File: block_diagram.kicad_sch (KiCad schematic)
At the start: 0 parts

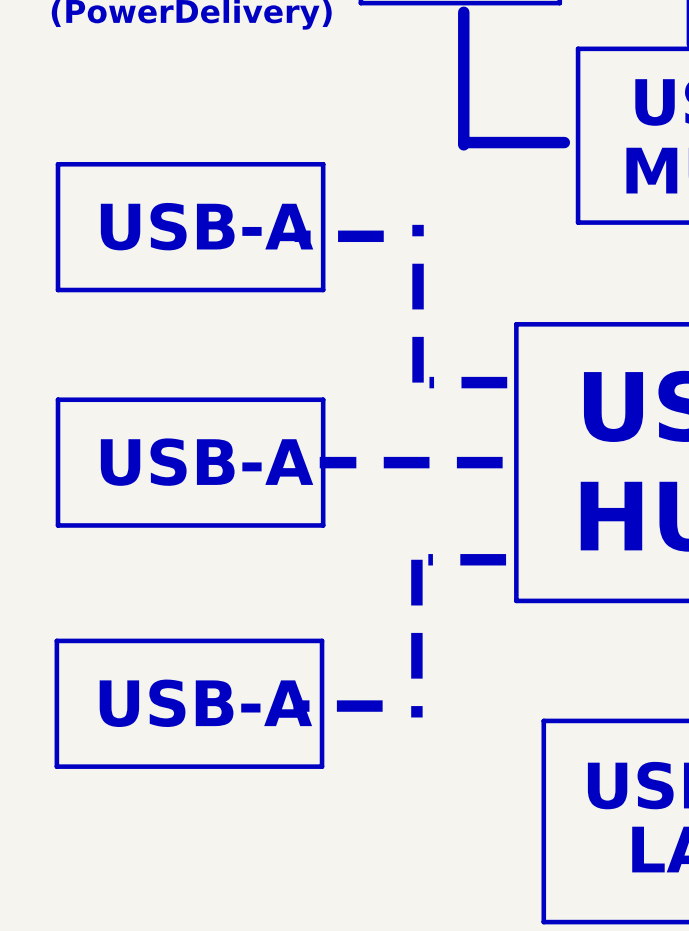
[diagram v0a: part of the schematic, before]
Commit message: Add files via upload
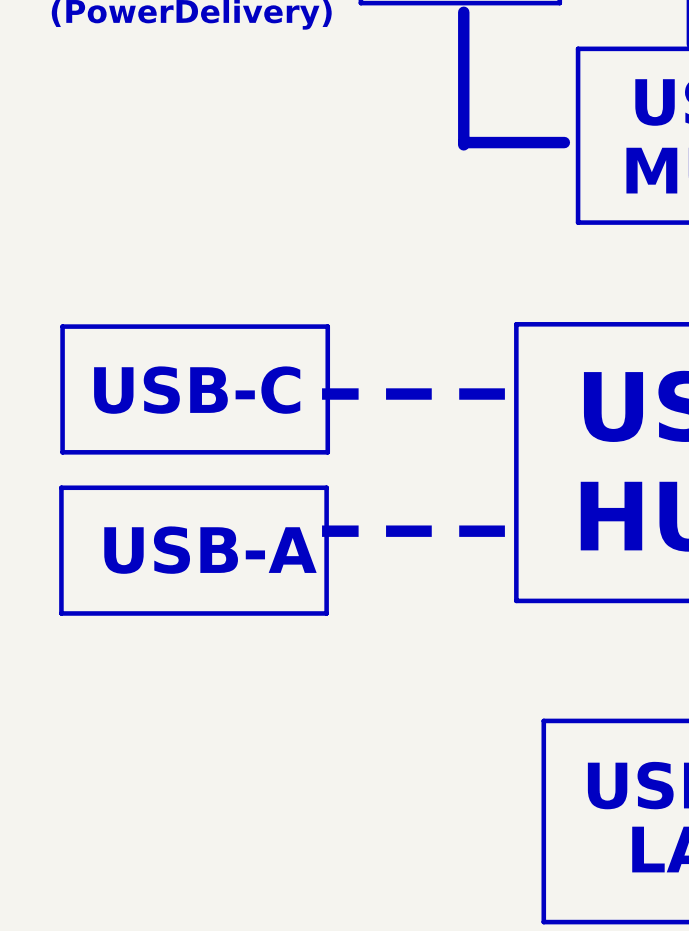
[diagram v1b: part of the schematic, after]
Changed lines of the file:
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@@
-	)
-	(rectangle
-		(start 62.103 84.963)
-		(end 91.567 98.933)
-		(stroke
-			(width 0.508)
-			(type solid)
-			(color 221 133 0 1)
-		)
-		(fill
-			(type none)
-		)
 	)
 	(rectangle
@@
 	)
 	(rectangle
-		(start 61.976 137.922)
-		(end 91.44 151.892)
+		(start 62.484 120.904)
+		(end 91.948 134.874)
 		(stroke
 			(width 0.508)
@@
 	)
 	(rectangle
-		(start 62.103 111.125)
-		(end 91.567 125.095)
+		(start 62.611 102.997)
+		(end 92.075 116.967)
 		(stroke
 			(width 0.508)
@@
 		)
 	)
+	(text "USB-C"
+		(exclude_from_sim no)
+		(at 77.47 110.49 0)
+		(effects
+			(font
+				(size 5.08 5.08)
+				(thickness 1.016)
+				(bold yes)
+				(color 221 133 0 1)
+			)
+		)
+	)
+	(text "HUB"
+		(exclude_from_sim no)
+		(at 131.826 124.587 0)
+		(effects
+			(font
+				(size 7.62 7.62)
+				(thickness 1.524)
+				(bold yes)
+				(color 255 153 0 1)
+			)
+		)
+	)
+	(text "LAN"
+		(exclude_from_sim no)
+		(at 133.096 161.544 0)
+		(effects
+			(font
+				(size 5.08 5.08)
+				(thickness 1.016)
+				(bold yes)
+				(color 132 0 132 1)
+			)
+		)
+	)
 	(text "USB-A "
 		(exclude_from_sim no)
-		(at 78.359 118.491 0)
-		(effects
-			(font
-				(size 5.08 5.08)
-				(thickness 1.016)
-				(bold yes)
-				(color 221 133 0 1)
-			)
-		)
-	)
-	(text "HUB"
-		(exclude_from_sim no)
-		(at 131.826 124.587 0)
-		(effects
-			(font
-				(size 7.62 7.62)
-				(thickness 1.524)
-				(bold yes)
-				(color 255 153 0 1)
-			)
-		)
-	)
-	(text "LAN"
-		(exclude_from_sim no)
-		(at 133.096 161.544 0)
-		(effects
-			(font
-				(size 5.08 5.08)
-				(thickness 1.016)
-				(bold yes)
-				(color 132 0 132 1)
-			)
-		)
-	)
-	(text "USB-A "
-		(exclude_from_sim no)
-		(at 78.232 145.288 0)
+		(at 78.74 128.27 0)
 		(effects
 			(font
@@
 		)
 	)
-	(text "USB-A "
-		(exclude_from_sim no)
-		(at 78.359 92.329 0)
-		(effects
-			(font
-				(size 5.08 5.08)
-				(thickness 1.016)
-				(bold yes)
-				(color 221 133 0 1)
-			)
-		)
-	)
 	(text "USB"
 		(exclude_from_sim no)
@@
 	(polyline
 		(pts
-			(xy 111.887 128.905) (xy 103.251 128.905)
+			(xy 221.361 134.239) (xy 209.423 134.239)
+		)
+		(stroke
+			(width 1.27)
+			(type solid)
+			(color 255 255 0 1)
+		)
+	)
+	(polyline
+		(pts
+			(xy 209.423 134.239) (xy 209.423 120.777)
+		)
+		(stroke
+			(width 1.27)
+			(type solid)
+			(color 255 255 0 1)
+		)
+	)
+	(polyline
+		(pts
+			(xy 163.957 81.788) (xy 148.209 81.788)
+		)
+		(stroke
+			(width 1.27)
+			(type solid)
+			(color 255 255 0 1)
+		)
+	)
+	(polyline
+		(pts
+			(xy 118.364 82.55) (xy 107.188 82.55)
+		)
+		(stroke
+			(width 1.27)
+			(type solid)
+			(color 255 255 0 1)
+		)
+	)
+	(polyline
+		(pts
+			(xy 111.76 125.73) (xy 91.44 125.73)
 		)
 		(stroke
@@
 	(polyline
 		(pts
-			(xy 221.361 134.239) (xy 209.423 134.239)
-		)
-		(stroke
-			(width 1.27)
-			(type solid)
-			(color 255 255 0 1)
-		)
-	)
-	(polyline
-		(pts
-			(xy 209.423 134.239) (xy 209.423 120.777)
-		)
-		(stroke
-			(width 1.27)
-			(type solid)
-			(color 255 255 0 1)
-		)
-	)
-	(polyline
-		(pts
-			(xy 101.981 128.905) (xy 101.981 146.431)
+			(xy 132.842 134.366) (xy 132.842 146.304)
 		)
 		(stroke
@@
 	(polyline
 		(pts
-			(xy 98.171 145.161) (xy 88.265 145.161)
+			(xy 209.423 120.777) (xy 204.851 120.777)
+		)
+		(stroke
+			(width 1.27)
+			(type solid)
+			(color 255 255 0 1)
+		)
+	)
+	(polyline
+		(pts
+			(xy 107.188 82.804) (xy 107.188 68.072)
+		)
+		(stroke
+			(width 1.27)
+			(type solid)
+			(color 255 255 0 1)
+		)
+	)
+	(polyline
+		(pts
+			(xy 111.76 110.49) (xy 91.44 110.49)
 		)
 		(stroke
@@
 	(polyline
 		(pts
-			(xy 163.957 81.788) (xy 148.209 81.788)
-		)
-		(stroke
-			(width 1.27)
-			(type solid)
-			(color 255 255 0 1)
-		)
-	)
-	(polyline
-		(pts
-			(xy 98.298 92.964) (xy 88.392 92.964)
-		)
-		(stroke
-			(width 1.27)
-			(type dot)
-			(color 255 255 0 1)
-		)
-	)
-	(polyline
-		(pts
-			(xy 118.364 82.55) (xy 107.188 82.55)
-		)
-		(stroke
-			(width 1.27)
-			(type solid)
-			(color 255 255 0 1)
-		)
-	)
-	(polyline
-		(pts
-			(xy 112.014 109.22) (xy 103.378 109.22)
-		)
-		(stroke
-			(width 1.27)
-			(type dot)
-			(color 255 255 0 1)
-		)
-	)
-	(polyline
-		(pts
-			(xy 132.842 134.366) (xy 132.842 146.304)
-		)
-		(stroke
-			(width 1.27)
-			(type dot)
-			(color 255 255 0 1)
-		)
-	)
-	(polyline
-		(pts
-			(xy 209.423 120.777) (xy 204.851 120.777)
-		)
-		(stroke
-			(width 1.27)
-			(type solid)
-			(color 255 255 0 1)
-		)
-	)
-	(polyline
-		(pts
-			(xy 107.188 82.804) (xy 107.188 68.072)
-		)
-		(stroke
-			(width 1.27)
-			(type solid)
-			(color 255 255 0 1)
-		)
-	)
-	(polyline
-		(pts
-			(xy 111.506 118.11) (xy 91.186 118.11)
-		)
-		(stroke
-			(width 1.27)
-			(type dot)
-			(color 255 255 0 1)
-		)
-	)
-	(polyline
-		(pts
 			(xy 132.842 102.108) (xy 132.842 93.218)
 		)
@@
 	(polyline
 		(pts
-			(xy 102.108 109.22) (xy 102.108 91.694)
-		)
-		(stroke
-			(width 1.27)
-			(type dot)
-			(color 255 255 0 1)
-		)
-	)
-	(polyline
-		(pts
 			(xy 209.55 114.046) (xy 204.978 114.046)
 		)
@@
 			(type solid)
 			(color 255 255 0 1)
-		)
-	)
-	(group ""
-		(members "20b66ea8-e42b-452b-8b2a-60ccbc024280" "2f185741-684f-4034-9a23-f1ae55aa6f8a"
-			"370711af-fc22-4f6a-b2e1-5d0cae1ba513"
 		)
 	)
@@
 		)
 	)
-	(group ""
-		(members "3c3c2c3c-84f3-4b08-9b6d-b1c3f04c1163" "4f0b2e39-2793-47c1-98c1-0b5c1257a466"
-			"c6861dce-283e-48e7-ae09-d7c5116278bb"
-		)
-	)
-	(group ""
-		(members "85484f0b-dd46-43e8-808b-f09e818f87dc" "d5905486-6bc7-4a8e-b3b3-c04a281e7152")
-	)
 )

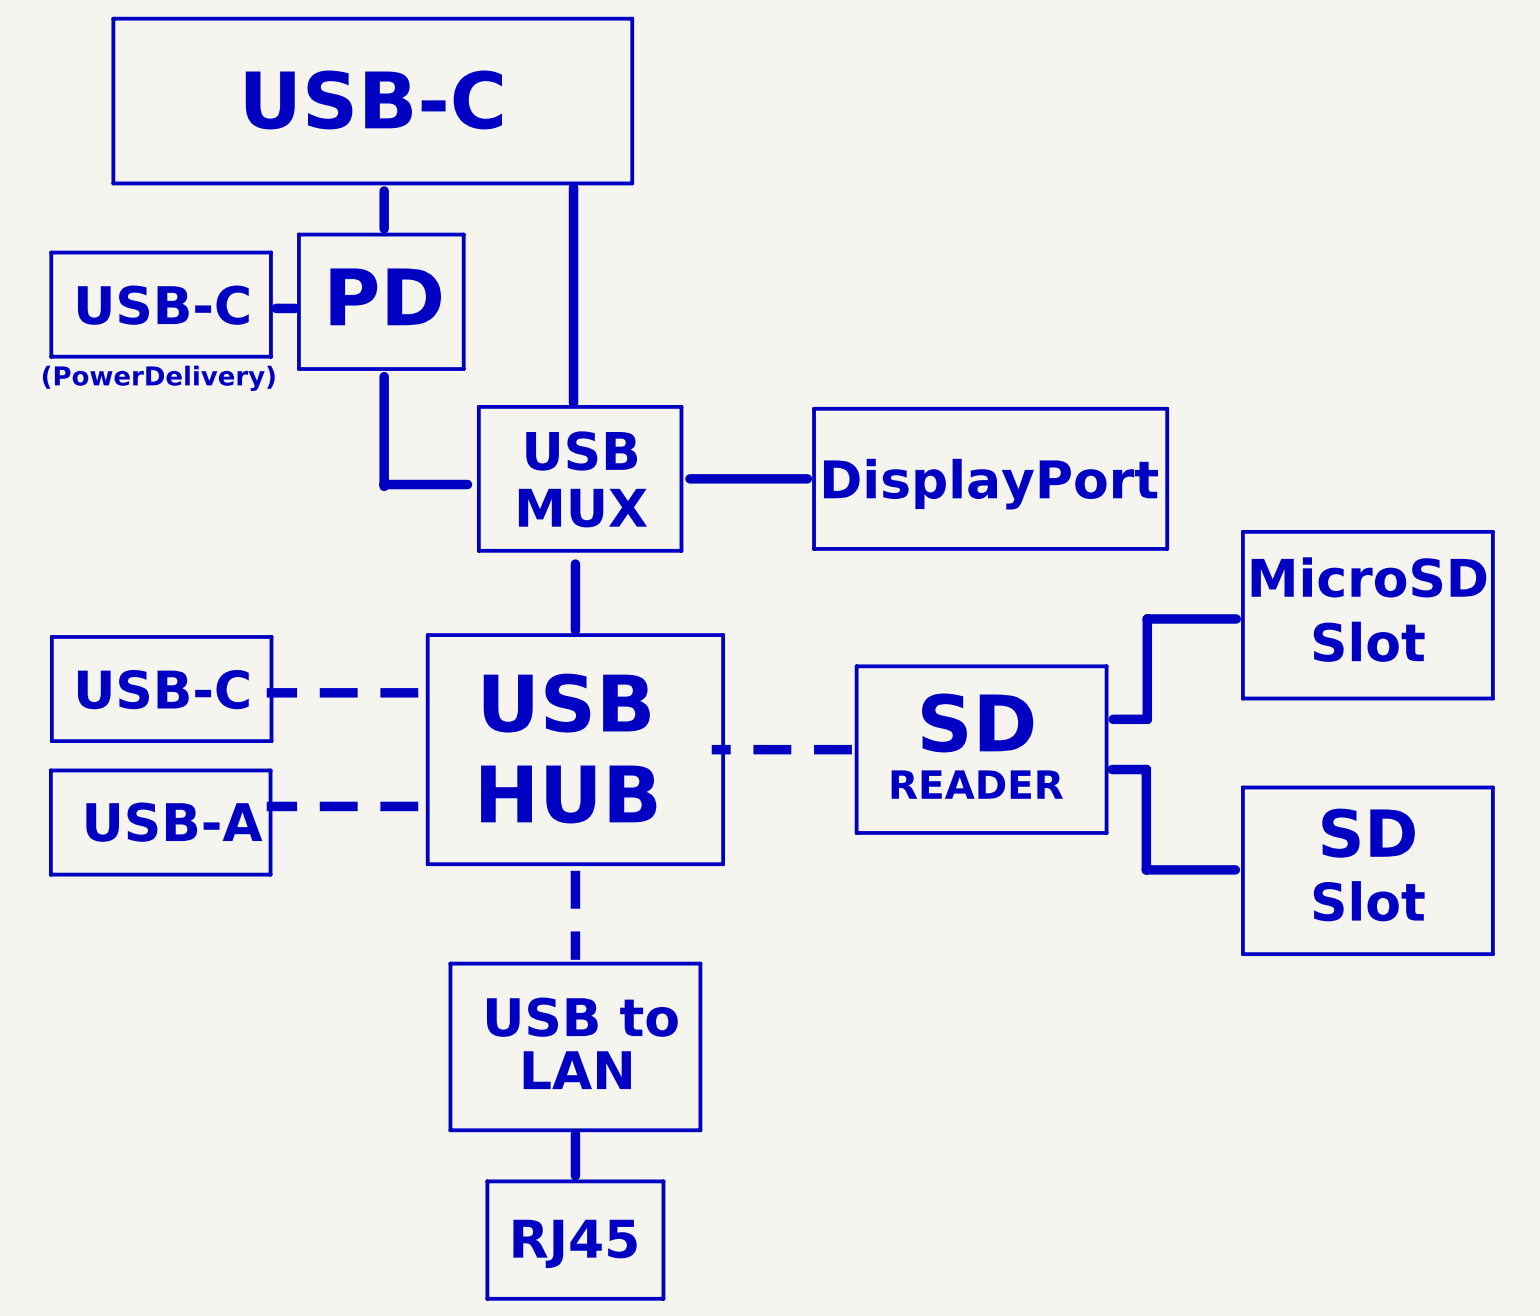
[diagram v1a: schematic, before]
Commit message: Add files via upload
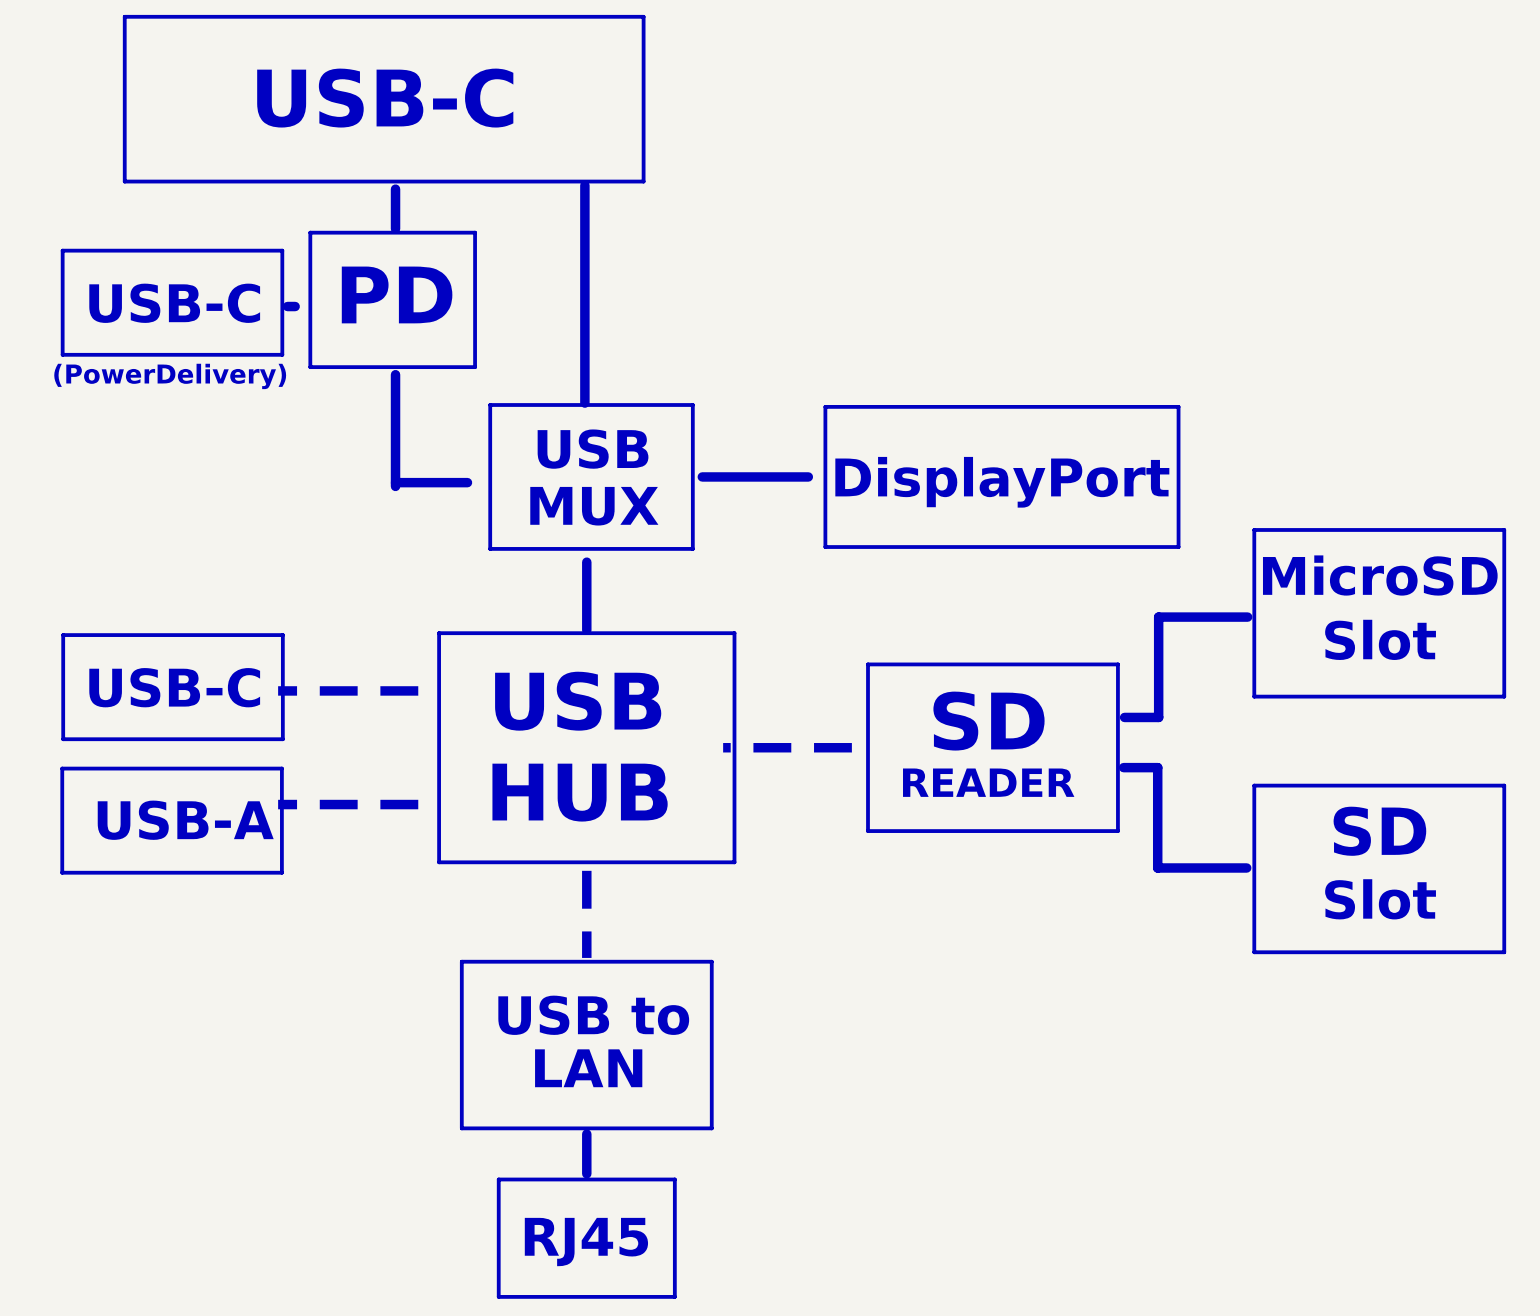
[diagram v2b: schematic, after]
